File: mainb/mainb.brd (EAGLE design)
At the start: 100 x 80 mm, 18 parts, among them IC1 REG1117, U1 ATTINY2313A

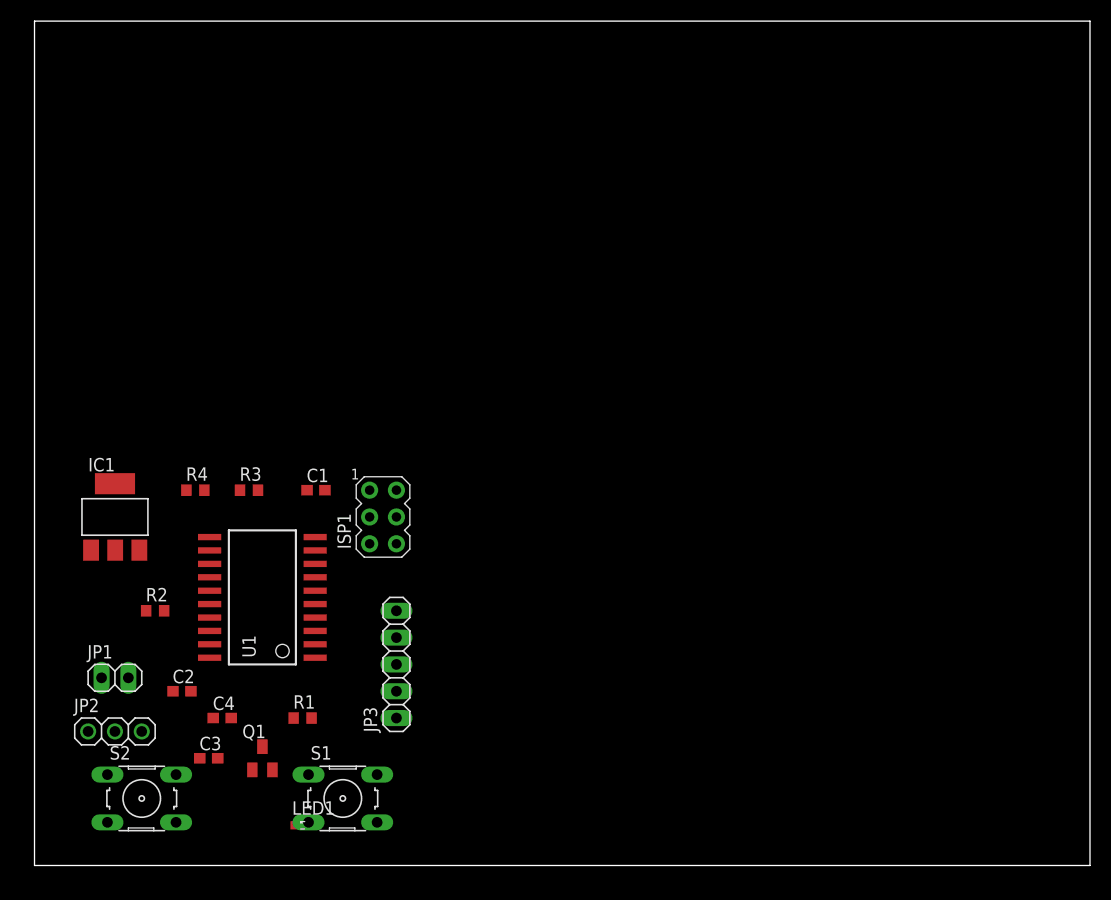
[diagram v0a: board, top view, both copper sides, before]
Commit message: added sunil stuff and playing around with eagle etc
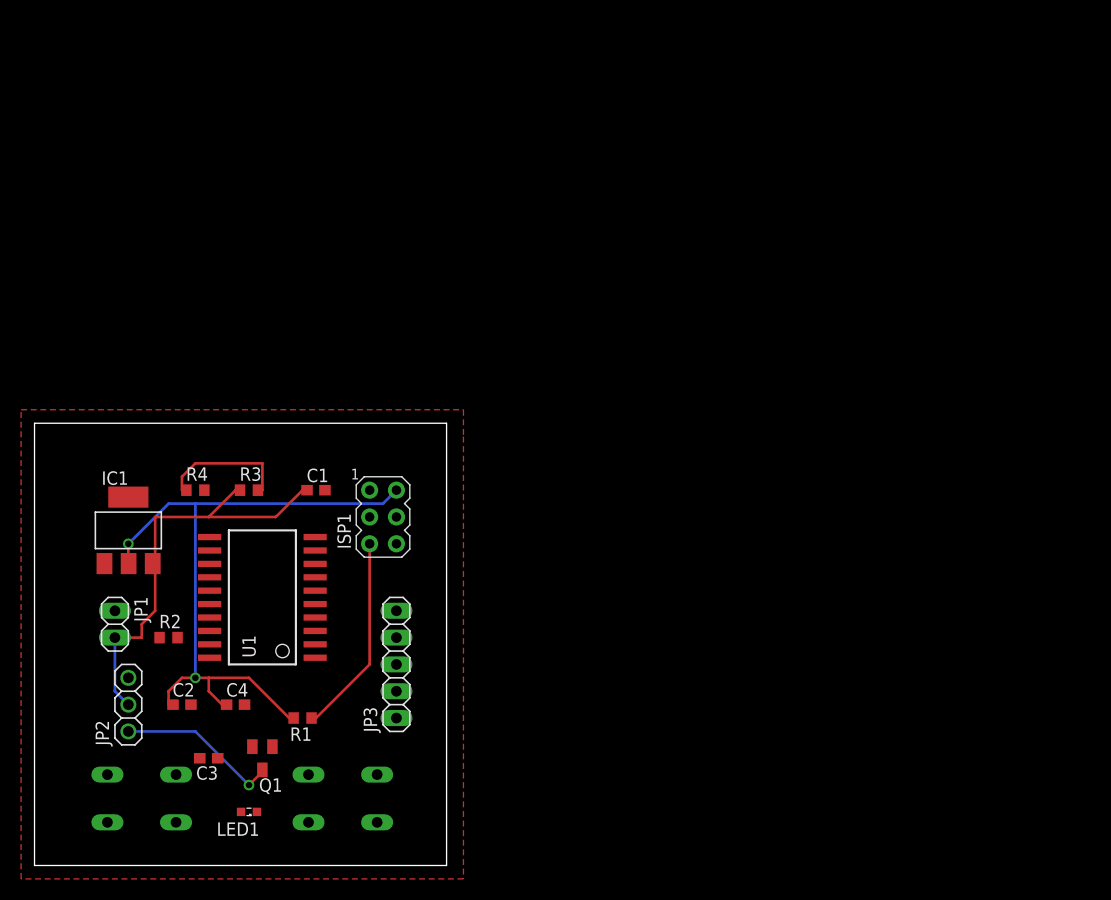
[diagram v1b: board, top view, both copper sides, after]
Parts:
- moved LED1 5.24 mm to (20.3, 5.08), turned to 180 degrees
- moved JP1 5.08 mm to (7.62, 22.9), turned to 270 degrees
- moved JP2 2.84 mm to (8.89, 15.2), turned to 90 degrees
- moved R2 2.84 mm to (12.7, 21.6)
- moved IC1 1.80 mm to (8.89, 31.8)
- moved C4 1.80 mm to (19.1, 15.2)
- moved C2 1.27 mm to (14.0, 15.2)
- turned C3 to 180 degrees
- turned Q1 to 180 degrees
- turned R1 to 180 degrees
- flipped S1 to the bottom
- flipped S2 to the bottom
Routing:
- net ISP2: track 0.00 -> 65.0 mm, vias 0 -> 2
- net +5V: track 0.00 -> 40.9 mm
- net ISP5: track 0.00 -> 19.0 mm
- net N$1: track 0.00 -> 15.5 mm, vias 0 -> 1
- net N$10: track 0.00 -> 12.8 mm
- added copper zone on layer 1, net GND
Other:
- board size 100 x 80 mm -> 39 x 41.9 mm
